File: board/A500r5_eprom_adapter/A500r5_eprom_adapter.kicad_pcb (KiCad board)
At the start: 2 copper layers, 10 parts, among them J1 PWR, J2 A18 Selector, J3 A19 Selector, U1 27C400-A500, U2 27C080-L, U3 27C080-L

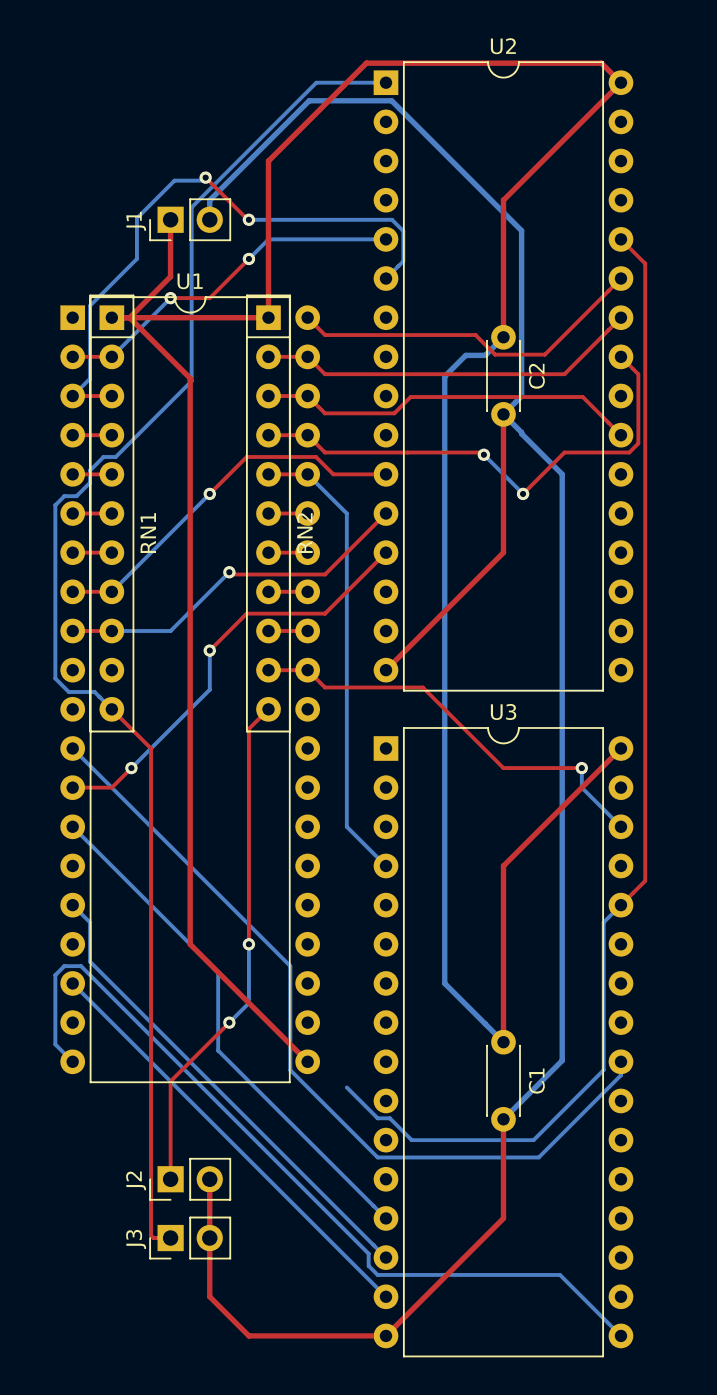
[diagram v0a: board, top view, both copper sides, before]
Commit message: More changes to the circuit
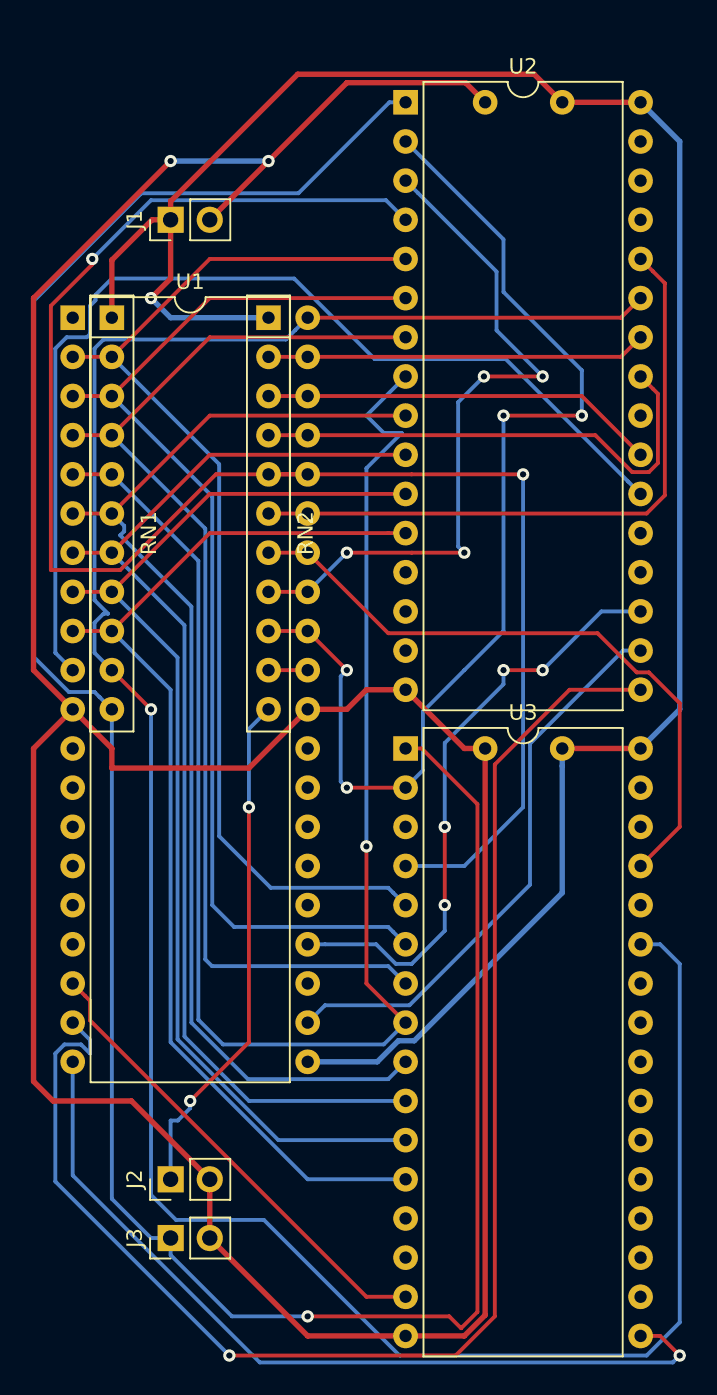
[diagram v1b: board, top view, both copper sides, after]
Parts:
- C1, C2: moved to B.Cu
- moved C1 19.4 mm to (138.4, 99.1), turned to 180 degrees
- moved C2 15.7 mm to (138.4, 57.1), turned to 180 degrees
- moved U2 1.80 mm to (128.3, 57.1)
- moved U3 1.27 mm to (128.3, 99.1)
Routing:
- net /A8: track 23.4 -> 159.9 mm, vias 0 -> 1
- net /A4: track 2.54 -> 101.5 mm, vias 0 -> 1
- net /D3-L: track 0.00 -> 95.0 mm, vias 0 -> 1
- net /A12: track 30.0 -> 110.2 mm, vias 0 -> 2
- net /A3: track 2.54 -> 75.5 mm
- net /A5: track 2.54 -> 74.4 mm
- net /A2: track 2.54 -> 73.6 mm
- net /A16: track 2.54 -> 72.2 mm, vias 0 -> 4
- net /~CE: track 0.00 -> 68.2 mm
- net /A19: track 92.1 -> 158.1 mm, vias 0 -> 1
- net VCC: track 199.5 -> 137.7 mm, vias 0 -> 1
- net GND: track 146.0 -> 202.3 mm, vias 0 -> 2
- net /~OE: track 53.6 -> 0.00 mm
- net /A7: track 23.5 -> 72.1 mm, vias 2 -> 0
- net /A1: track 24.4 -> 72.5 mm, vias 1 -> 0
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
